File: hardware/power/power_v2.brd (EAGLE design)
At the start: 92 x 92 mm, 59 parts, among them J1 FASTON1289_ST, J2 FASTON1289_ST, J3 12v, J4 5v, J5 XT30PW-F, J6 XT30PW-F, J7 XT30PW-F, J8 XT30PW-F, Q1 MMBT5401L, Q2 PSMN1R0-40YSH, Q3 MMBT5401L, Q4 PSMN1R0-40YSH, U1 PDQ30-Q24-S5-D, U2 PDQ30-Q24-S12-D

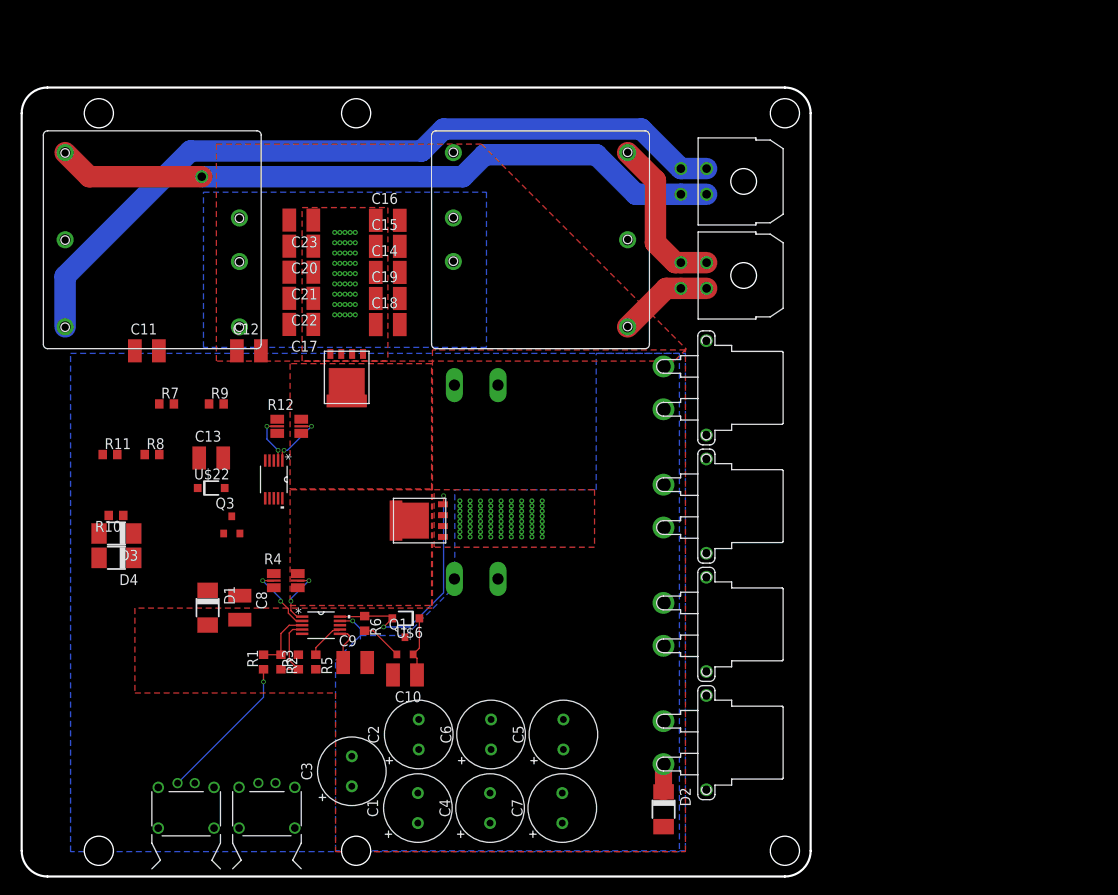
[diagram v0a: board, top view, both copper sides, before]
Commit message: Another repeat redo
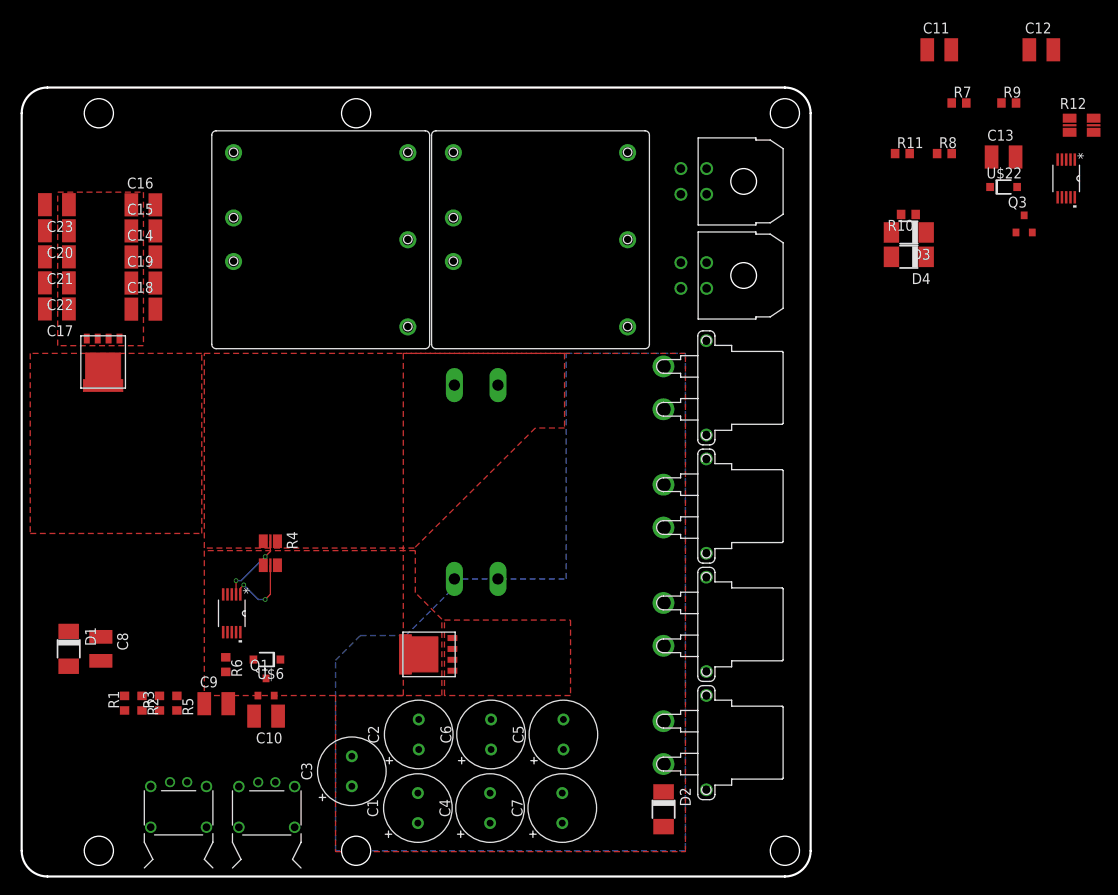
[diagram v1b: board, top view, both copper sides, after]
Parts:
- moved C11 98.8 mm to (107.0, 96.4)
- moved C12 98.8 mm to (118.9, 96.4)
- moved C13 98.8 mm to (114.5, 83.9)
- moved Q3 98.8 mm to (116.9, 76.1)
- moved R10 98.8 mm to (103.4, 77.2)
- moved R11 98.8 mm to (102.7, 84.3)
- moved R7 98.8 mm to (109.3, 90.2)
- moved U$14 98.8 mm to (121.8, 81.4)
- moved U$22 98.8 mm to (114.5, 80.4)
- moved D3 98.8 mm to (103.4, 75.1)
- moved D4 98.8 mm to (103.4, 72.3)
- moved R12 98.8 mm to (123.6, 87.6)
- moved R8 98.8 mm to (107.6, 84.3)
- moved R9 98.8 mm to (115.1, 90.2)
- moved C14 28.6 mm to (14.2, 72.2)
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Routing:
- net 12V_GND: track 89.7 -> 0.00 mm
- net +12VOUT: track 78.9 -> 0.00 mm, vias 1 -> 0
- net N$5: track 28.7 -> 0.00 mm, vias 2 -> 0
- net 5V_GND: track 18.8 -> 0.00 mm
- net N$3: track 17.4 -> 0.00 mm, vias 1 -> 0
- net +5VOUT: track 11.1 -> 0.00 mm
- net N$2: track 8.39 -> 0.00 mm
- net N$1: track 7.38 -> 0.00 mm
- net +24V_LEG: track 7.21 -> 0.00 mm, vias 73 -> 0
- net N$8: track 7.09 -> 0.00 mm
- net N$20: track 6.84 -> 0.00 mm, vias 2 -> 0
- net N$19: track 5.74 -> 0.00 mm, vias 2 -> 0
- net N$9: track 4.89 -> 0.00 mm
- net N$7: track 4.62 -> 0.00 mm
- net N$6: track 4.51 -> 0.00 mm
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- added copper zone on layer 1, net +24V_BATT
- removed copper zone on layer 16, net +24V_BATT
- removed copper zone on layer 16, net +24V_ISO

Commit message: Happy with this layout
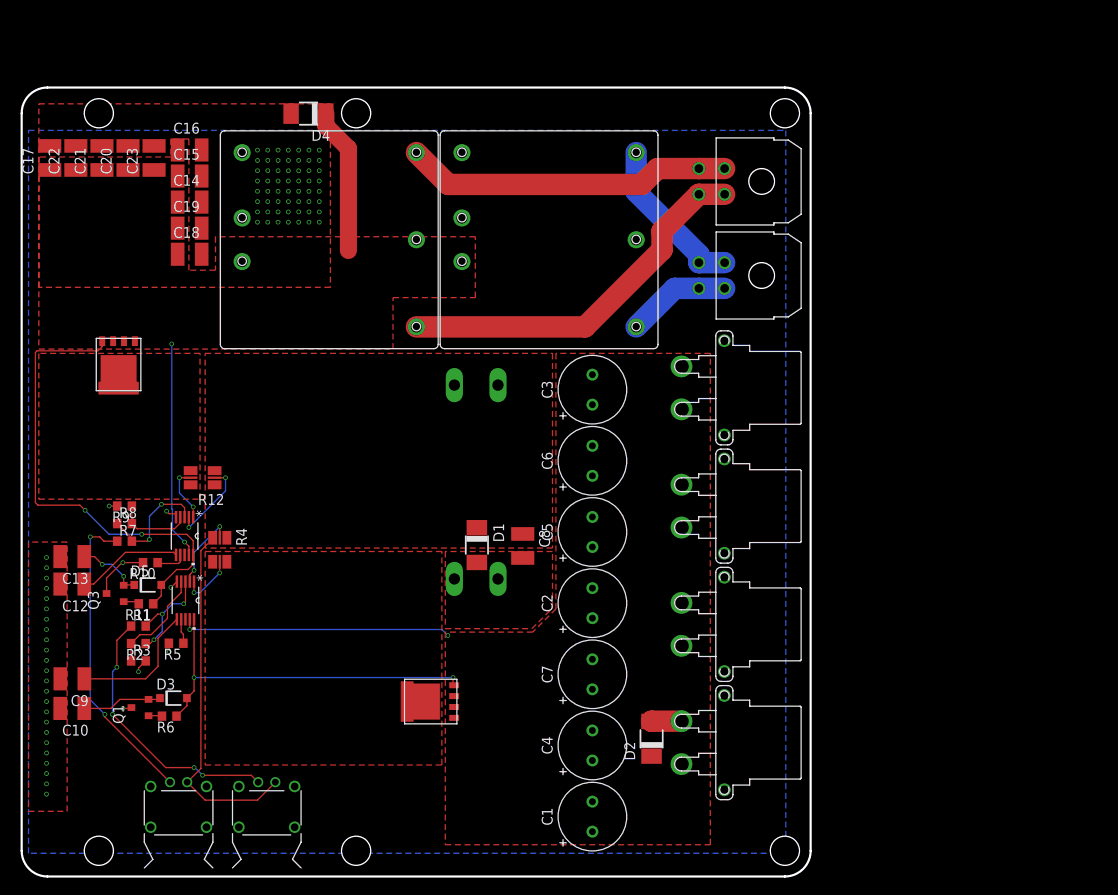
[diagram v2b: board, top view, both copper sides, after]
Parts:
- removed C11: 0.01uF, timlib:C1210
- removed U$22, U$6: 1N4148W-7-F, timlib:SOD123
- added D5: 1N4148W-7-F, timlib:SOD123
- D3: value SMAJ30A -> 1N4148W-7-F; device timlib:DO-214AC -> timlib:SOD123
- moved C12 129.0 mm to (5.90, 34.1), turned to 180 degrees
- moved C13 118.2 mm to (5.90, 37.3), turned to 180 degrees
- moved Q3 114.4 mm to (10.9, 33.0), turned to 90 degrees
- moved R9 113.3 mm to (12.0, 43.2), turned to 180 degrees
- moved U$14 110.9 mm to (19.0, 39.7)
- moved R12 110.4 mm to (21.1, 46.5), turned to 180 degrees
- moved R7 109.9 mm to (12.0, 39.1)
- moved R8 104.9 mm to (12.0, 41.1)
- moved R11 102.6 mm to (14.5, 31.8), turned to 180 degrees
- moved D3 101.5 mm to (17.7, 20.8), turned to 0 degrees
- moved R10 97.3 mm to (15.0, 36.6)
- moved D4 72.0 mm to (33.4, 89.0)
- moved C3 52.6 mm to (66.6, 56.8)
- moved C8 50.6 mm to (58.4, 38.5)
- moved D1 49.1 mm to (53.1, 38.6)
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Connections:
- net +24V_BATT: no longer C11.1, D3.C
- net GND_BATT: no longer C11.2, D3.A
- net N$14: now also D5.A; no longer U$22.A
- net N$17: now also D5.C; no longer U$22.C
- net N$5: now also D3.A; no longer U$6.A
- net N$8: now also D3.C; no longer U$6.C
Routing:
- net N$14: track 0.00 -> 56.5 mm, vias 0 -> 2
- net +12VOUT: track 0.00 -> 43.6 mm
- net N$5: track 0.00 -> 43.3 mm, vias 0 -> 2
- net +24V_ISO: track 0.00 -> 42.5 mm, vias 0 -> 2
- net +24V_BATT: track 0.00 -> 40.8 mm
- net 12V_GND: track 0.00 -> 38.2 mm
- net N$13: track 0.00 -> 35.8 mm, vias 0 -> 2
- net +24V_LEG: track 0.00 -> 31.6 mm, vias 0 -> 2
- net N$3: track 0.00 -> 31.4 mm, vias 0 -> 4
- net 5V_GND: track 0.00 -> 18.9 mm
- net GND_BATT: track 0.00 -> 17.5 mm, vias 0 -> 87
- net N$7: track 0.00 -> 15.6 mm
- net N$4: track 0.00 -> 13.5 mm, vias 0 -> 2
- net N$1: track 0.00 -> 12.7 mm, vias 0 -> 3
- net N$2: track 0.00 -> 12.4 mm
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- added copper zone on layer 16, net GND_BATT
- removed copper zone on layer 16, net +24V_LEG
